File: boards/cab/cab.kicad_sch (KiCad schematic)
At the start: 44 parts, among them J1 Conn_01x08_Female, J2 Conn_01x08_Female, J3 Conn_01x08_Female, J4 Conn_01x08_Female, Q1 SI2308A, Q2 S8550, Q3 BC817-40,215, Q4 S8550, Q5 BC817-40,215, Q6 S8550, Q7 BC817-40,215, Q8 S8550, SW1 SW_Push, U1 XL1509-ADJ, U2 XL1509-5.0, U3 ATTINY1616-MNR

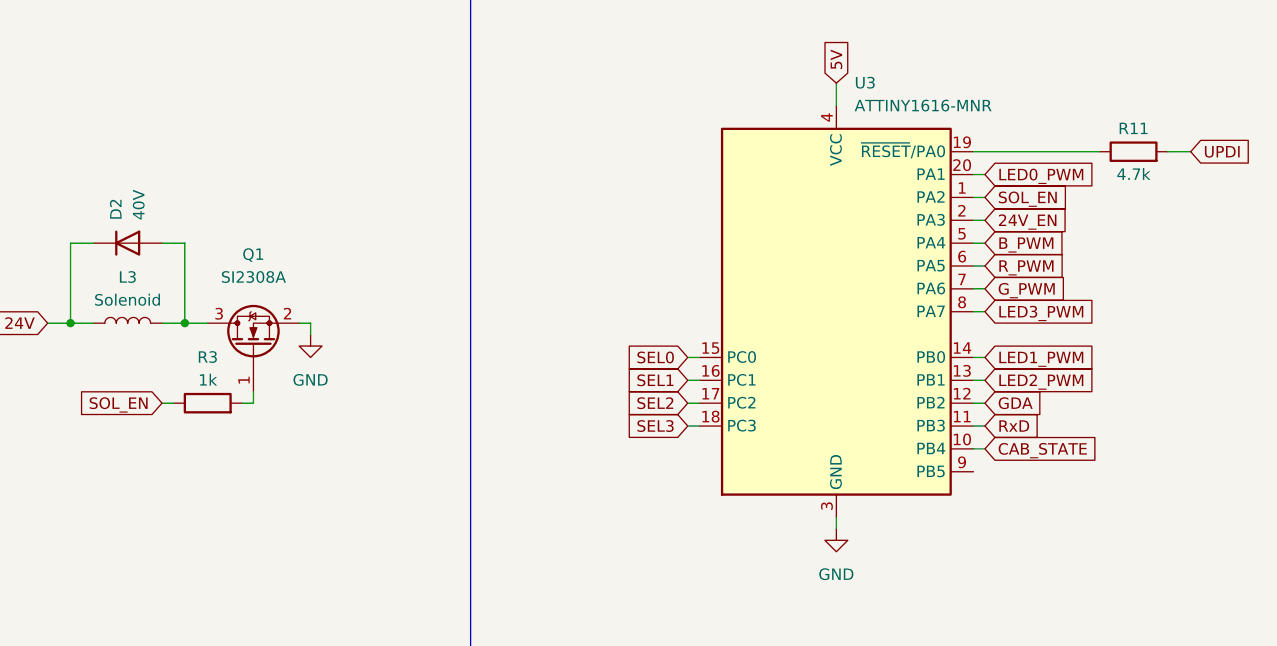
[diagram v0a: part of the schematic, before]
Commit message: Routing & planes
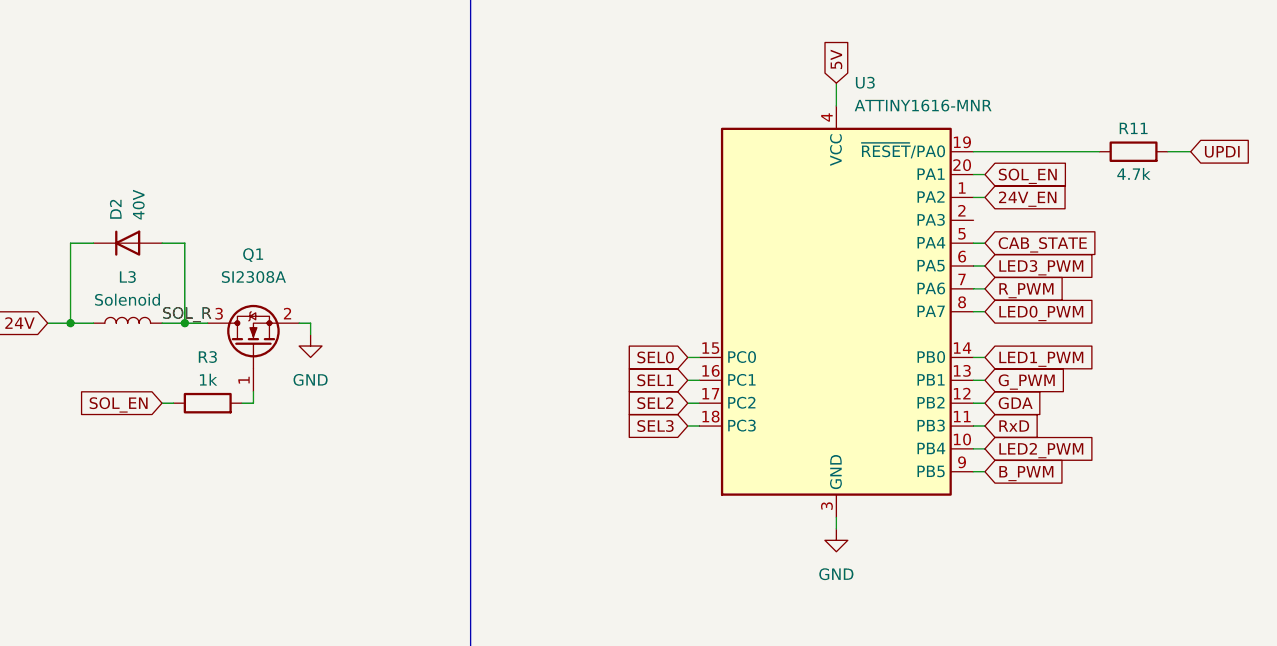
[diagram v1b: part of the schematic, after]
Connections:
- net 24V_EN: now also U3.1 (PA2); no longer U3.2 (PA3)
- net B_PWM: now also U3.9 (PB5); no longer U3.5 (PA4)
- net CAB_STATE: now also U3.5 (PA4); no longer U3.10 (PB4)
- net G_PWM: now also U3.13 (PB1); no longer U3.7 (PA6)
- net LED0_PWM: now also U3.8 (PA7); no longer U3.20 (PA1)
- net LED2_PWM: now also U3.10 (PB4); no longer U3.13 (PB1)
- net LED3_PWM: now also U3.6 (PA5); no longer U3.8 (PA7)
- net R_PWM: now also U3.7 (PA6); no longer U3.6 (PA5)
- net SOL_EN: now also U3.20 (PA1); no longer U3.1 (PA2)
- net SOL_R: now reaches D2.2 (A), L3.2, Q1.3 (D)
